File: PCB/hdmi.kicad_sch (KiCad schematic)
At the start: 25 parts, among them J7 HDMI_D_1.4, U12 PCA9306DC1, U14 UCL0524P, U15 UCL0524P, U16 UCL0524P

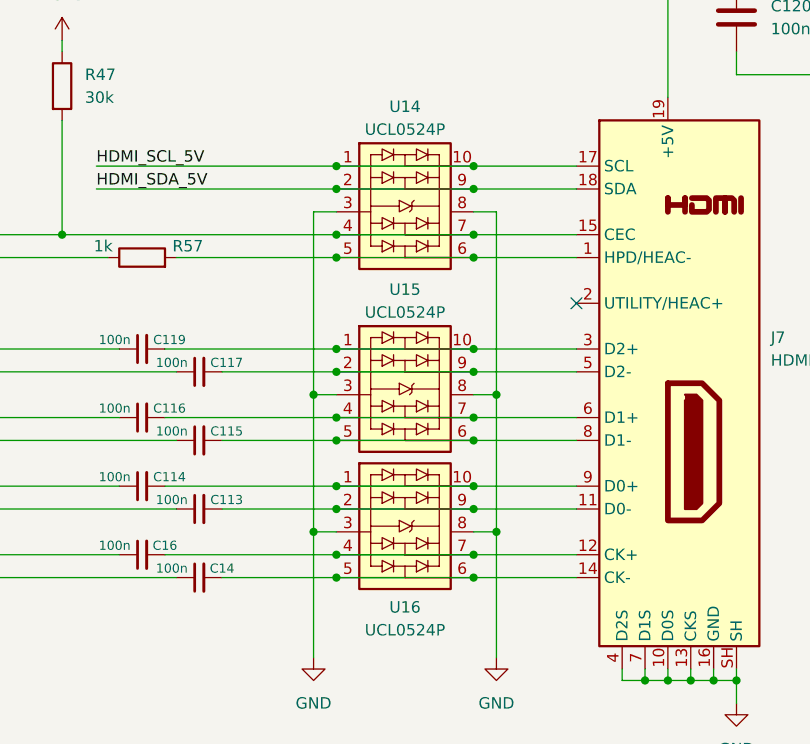
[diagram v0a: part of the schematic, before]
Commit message: a bunch of stuff!
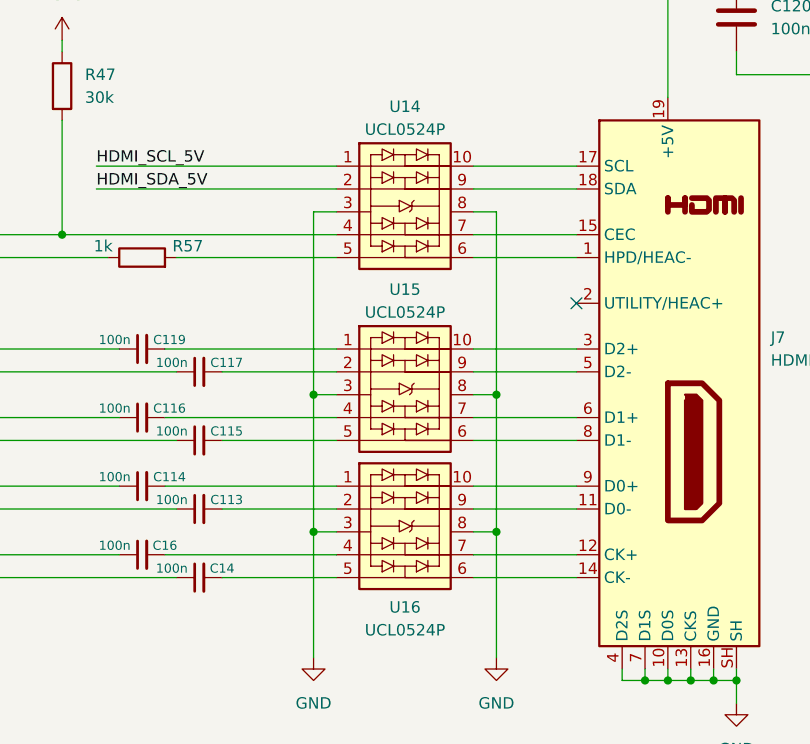
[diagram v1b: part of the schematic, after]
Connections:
- net HDMI_CEC: no longer J7.15 (CEC), U14.7
- net HDMI_SCL_5V: no longer J7.17 (SCL), U14.10
- net HDMI_SDA_5V: no longer J7.18 (SDA), U14.9
- net at R57.2, U14.5: no longer J7.1 (HPD/HEAC-), U14.6
- net at C117.2, U15.2: no longer J7.5 (D2-), U15.9
- net at C116.2, U15.4: no longer J7.6 (D1+), U15.7
- net at C114.2, U16.1: no longer J7.9 (D0+), U16.10
- net at J7.11 (D0-), U16.9: no longer C113.2, U16.2
- net at J7.12 (CK+), U16.7: no longer C16.2, U16.4
- net at J7.14 (CK-), U16.6: no longer C14.2, U16.5
- net at J7.3 (D2+), U15.10: no longer C119.2, U15.1
- net at J7.8 (D1-), U15.6: no longer C115.2, U15.5
- new net: J7.1 (HPD/HEAC-), U14.6
- new net: J7.15 (CEC), U14.7
- new net: J7.17 (SCL), U14.10
- new net: J7.18 (SDA), U14.9
- new net: J7.5 (D2-), U15.9
- new net: J7.6 (D1+), U15.7
- new net: J7.9 (D0+), U16.10
- new net: C119.2, U15.1
- new net: C115.2, U15.5
- new net: C113.2, U16.2
- new net: C16.2, U16.4
- new net: C14.2, U16.5
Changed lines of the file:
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@@
-	)
-	(junction
-		(at 86.36 88.9)
-		(diameter 0)
-		(color 0 0 0 0)
 	)
 	(junction
@@
 	)
 	(junction
-		(at 86.36 109.22)
-		(diameter 0)
-		(color 0 0 0 0)
-	)
-	(junction
 		(at 130.81 146.05)
 		(diameter 0)
@@
 	)
 	(junction
-		(at 101.6 119.38)
-		(diameter 0)
-		(color 0 0 0 0)
-	)
-	(junction
-		(at 86.36 91.44)
-		(diameter 0)
-		(color 0 0 0 0)
-	)
-	(junction
-		(at 86.36 134.62)
-		(diameter 0)
-		(color 0 0 0 0)
-	)
-	(junction
 		(at 120.65 146.05)
 		(diameter 0)
@@
 	)
 	(junction
-		(at 101.6 124.46)
-		(diameter 0)
-		(color 0 0 0 0)
-	)
-	(junction
 		(at 251.46 96.52)
 		(diameter 0)
@@
 	)
 	(junction
-		(at 101.6 88.9)
-		(diameter 0)
-		(color 0 0 0 0)
-	)
-	(junction
 		(at 143.51 78.74)
 		(diameter 0)
@@
 	)
 	(junction
-		(at 101.6 127)
-		(diameter 0)
-		(color 0 0 0 0)
-	)
-	(junction
 		(at 83.82 114.3)
 		(diameter 0)
@@
 	)
 	(junction
-		(at 101.6 99.06)
-		(diameter 0)
-		(color 0 0 0 0)
-	)
-	(junction
-		(at 86.36 124.46)
-		(diameter 0)
-		(color 0 0 0 0)
-	)
-	(junction
-		(at 101.6 132.08)
-		(diameter 0)
-		(color 0 0 0 0)
-	)
-	(junction
-		(at 101.6 96.52)
-		(diameter 0)
-		(color 0 0 0 0)
-	)
-	(junction
-		(at 86.36 119.38)
-		(diameter 0)
-		(color 0 0 0 0)
-	)
-	(junction
-		(at 101.6 109.22)
-		(diameter 0)
-		(color 0 0 0 0)
-	)
-	(junction
-		(at 86.36 132.08)
-		(diameter 0)
-		(color 0 0 0 0)
-	)
-	(junction
 		(at 182.88 96.52)
 		(diameter 0)
@@
 	)
 	(junction
-		(at 86.36 96.52)
-		(diameter 0)
-		(color 0 0 0 0)
-	)
-	(junction
-		(at 86.36 111.76)
-		(diameter 0)
-		(color 0 0 0 0)
-	)
-	(junction
 		(at 104.14 114.3)
 		(diameter 0)
@@
 	)
 	(junction
-		(at 101.6 111.76)
-		(diameter 0)
-		(color 0 0 0 0)
-	)
-	(junction
 		(at 191.77 96.52)
 		(diameter 0)
@@
 	)
 	(junction
-		(at 86.36 116.84)
-		(diameter 0)
-		(color 0 0 0 0)
-	)
-	(junction
-		(at 101.6 91.44)
-		(diameter 0)
-		(color 0 0 0 0)
-	)
-	(junction
 		(at 83.82 129.54)
 		(diameter 0)
@@
 	)
 	(junction
-		(at 86.36 99.06)
-		(diameter 0)
-		(color 0 0 0 0)
-	)
-	(junction
 		(at 182.88 111.76)
 		(diameter 0)
@@
 	)
 	(junction
-		(at 101.6 134.62)
-		(diameter 0)
-		(color 0 0 0 0)
-	)
-	(junction
-		(at 101.6 116.84)
-		(diameter 0)
-		(color 0 0 0 0)
-	)
-	(junction
 		(at 130.81 66.04)
-		(diameter 0)
-		(color 0 0 0 0)
-	)
-	(junction
-		(at 86.36 127)
 		(diameter 0)
 		(color 0 0 0 0)
@@
 	(wire
 		(pts
-			(xy 86.36 124.46) (xy 101.6 124.46)
-		)
-		(stroke
-			(width 0)
-			(type default)
-		)
-	)
-	(wire
-		(pts
 			(xy 55.88 74.93) (xy 55.88 76.2)
 		)
@@
 	(wire
 		(pts
-			(xy 86.36 109.22) (xy 101.6 109.22)
-		)
-		(stroke
-			(width 0)
-			(type default)
-		)
-	)
-	(wire
-		(pts
 			(xy 101.6 88.9) (xy 113.03 88.9)
 		)
@@
 	(wire
 		(pts
-			(xy 86.36 132.08) (xy 101.6 132.08)
-		)
-		(stroke
-			(width 0)
-			(type default)
-		)
-	)
-	(wire
-		(pts
 			(xy 83.82 93.98) (xy 83.82 114.3)
 		)
@@
 	(wire
 		(pts
-			(xy 86.36 127) (xy 101.6 127)
-		)
-		(stroke
-			(width 0)
-			(type default)
-		)
-	)
-	(wire
-		(pts
 			(xy 191.77 107.95) (xy 191.77 114.3)
 		)
@@
 	(wire
 		(pts
-			(xy 86.36 96.52) (xy 101.6 96.52)
-		)
-		(stroke
-			(width 0)
-			(type default)
-		)
-	)
-	(wire
-		(pts
 			(xy 231.14 109.22) (xy 231.14 96.52)
 		)
@@
 	(wire
 		(pts
-			(xy 86.36 119.38) (xy 101.6 119.38)
-		)
-		(stroke
-			(width 0)
-			(type default)
-		)
-	)
-	(wire
-		(pts
 			(xy 55.88 96.52) (xy 86.36 96.52)
 		)
@@
 	(wire
 		(pts
-			(xy 86.36 88.9) (xy 101.6 88.9)
-		)
-		(stroke
-			(width 0)
-			(type default)
-		)
-	)
-	(wire
-		(pts
 			(xy 101.6 134.62) (xy 113.03 134.62)
 		)
@@
 	(wire
 		(pts
-			(xy 86.36 134.62) (xy 101.6 134.62)
-		)
-		(stroke
-			(width 0)
-			(type default)
-		)
-	)
-	(wire
-		(pts
 			(xy 219.71 125.73) (xy 219.71 124.46)
 		)
@@
 	(wire
 		(pts
-			(xy 86.36 111.76) (xy 101.6 111.76)
-		)
-		(stroke
-			(width 0)
-			(type default)
-		)
-	)
-	(wire
-		(pts
 			(xy 104.14 93.98) (xy 104.14 114.3)
 		)
@@
 	(wire
 		(pts
-			(xy 86.36 116.84) (xy 101.6 116.84)
-		)
-		(stroke
-			(width 0)
-			(type default)
-		)
-	)
-	(wire
-		(pts
 			(xy 35.56 116.84) (xy 62.23 116.84)
 		)
@@
 	(wire
 		(pts
-			(xy 86.36 99.06) (xy 101.6 99.06)
-		)
-		(stroke
-			(width 0)
-			(type default)
-		)
-	)
-	(wire
-		(pts
 			(xy 260.35 111.76) (xy 229.87 111.76)
 		)
@@
 		)
 		(stroke
-			(width 0)
-			(type default)
-		)
-	)
-	(wire
-		(pts
-			(xy 86.36 91.44) (xy 101.6 91.44)
-		)
-		(stroke
